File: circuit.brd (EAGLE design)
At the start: 141.9 x 72.4 mm, 13 parts, among them IC1 ATMEGA328-20P

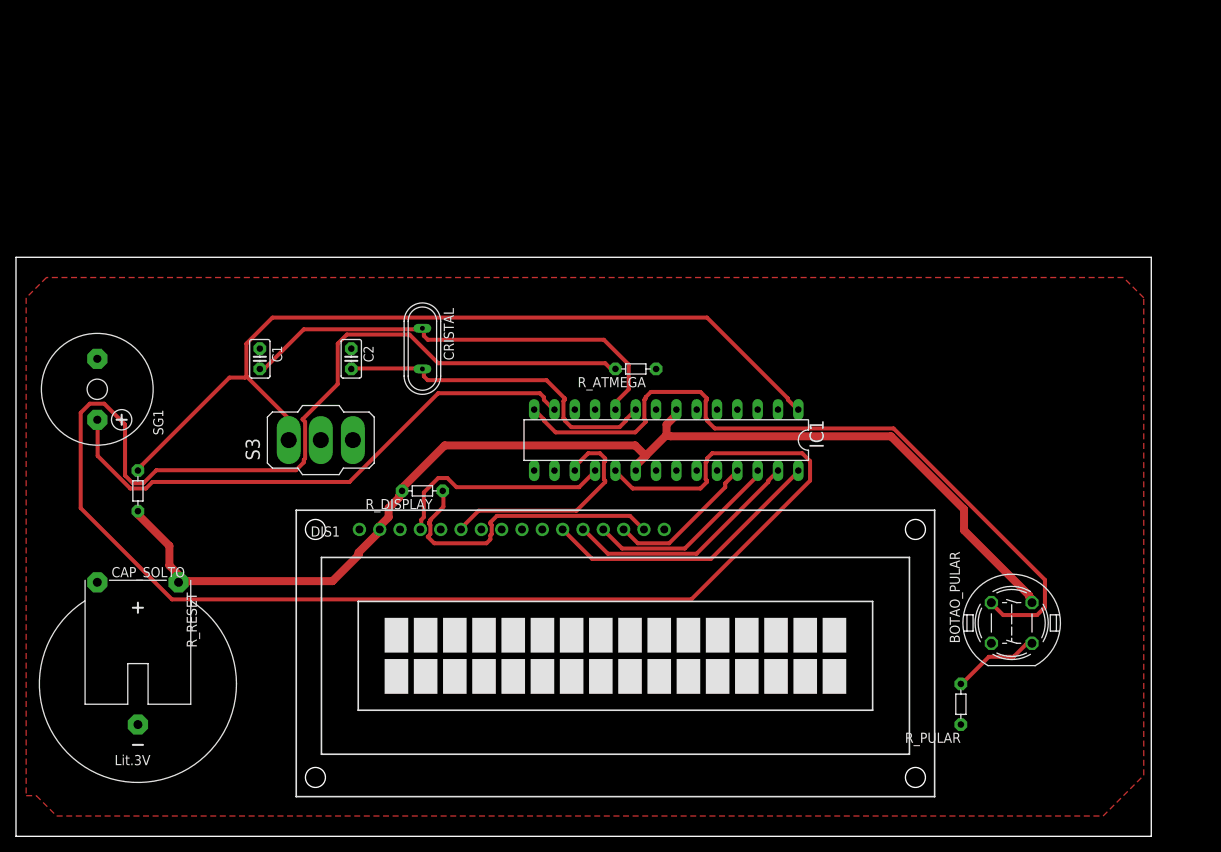
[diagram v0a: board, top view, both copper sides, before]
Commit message: Versão final do circuito
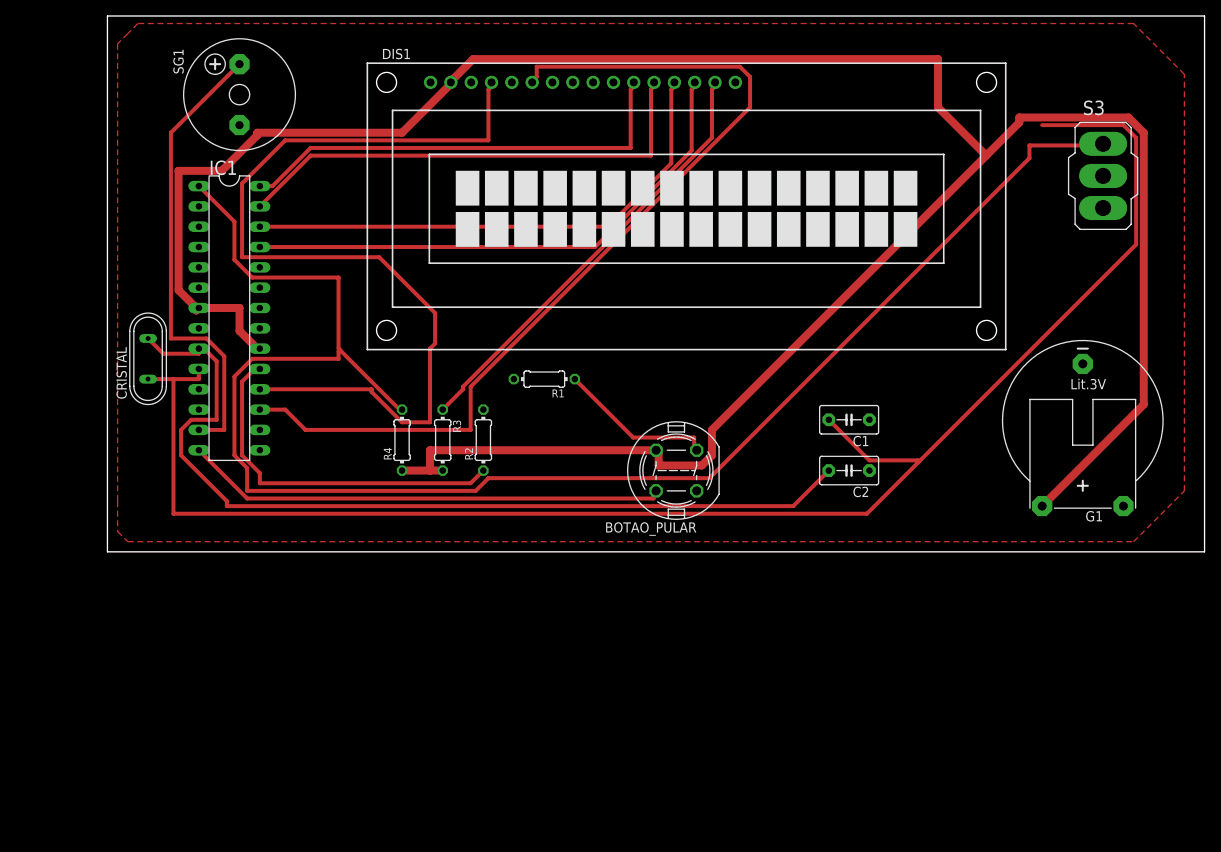
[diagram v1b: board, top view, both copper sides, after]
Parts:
- removed CAP_SOLTO: CR2430H, battery:CR2430H
- removed R_ATMEGA, R_DISPLAY, R_PULAR: (no value), discrete:R-5
- removed R_RESET: 10k, discrete:R-5
- added G1: CR2032H, battery:CR2032H
- added R1, R2, R3, R4: (no value), rcl:0204/7
- C1, C2: device capacitor-wima:C2.5-2 -> capacitor-wima:C5B3.5
- moved S3 103.2 mm to (133.3, 80.0), turned to 0 degrees
- moved C1 74.1 mm to (101.6, 49.5), turned to 180 degrees
- moved C2 63.8 mm to (101.6, 43.2), turned to 180 degrees
- moved IC1 56.7 mm to (24.1, 62.2), turned to 270 degrees
- moved DIS1 56.6 mm to (81.3, 76.2)
- moved BOTAO_PULAR 46.0 mm to (80.0, 43.2), turned to 180 degrees
- moved SG1 40.9 mm to (25.4, 90.2), turned to 90 degrees
- moved CRISTAL 34.3 mm to (14.0, 57.1), turned to 90 degrees
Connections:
- removed net N$7: IC1.19, R_ATMEGA.2
- removed net N$8: DIS1.15, R_DISPLAY.1
- new net N$2: IC1.19, R2.1
- new net N$3: DIS1.15, R3.1
- net GND: now also G1.-, R1.2, R2.2; no longer CAP_SOLTO.-, R_ATMEGA.1, R_PULAR.1
- net N$17: now also R1.1; no longer R_PULAR.2
- net N$4: now also R4.2; no longer R_RESET.1
- net VCC: now also G1.+, R3.2, R4.1; no longer CAP_SOLTO.+, R_DISPLAY.2, R_RESET.2
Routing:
- net N$7: track 236.9 -> 0.00 mm
- net VCC: track 144.8 -> 317.4 mm
- net N$5: track 56.8 -> 197.9 mm
- net N$4: track 108.0 -> 201.0 mm
- net N$10: track 29.0 -> 115.5 mm
- net N$9: track 28.3 -> 113.7 mm
- net N$6: track 41.8 -> 111.8 mm
- net N$3: track 0.00 -> 55.0 mm
- net N$15: track 19.0 -> 67.6 mm
- net N$2: track 0.00 -> 45.1 mm
- net N$13: track 24.7 -> 65.0 mm
- net N$8: track 37.6 -> 0.00 mm
- net N$19: track 91.9 -> 60.4 mm
- net N$12: track 30.1 -> 60.8 mm
- net N$11: track 35.7 -> 56.7 mm
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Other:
- board size 141.9 x 72.4 mm -> 137.1 x 67 mm
